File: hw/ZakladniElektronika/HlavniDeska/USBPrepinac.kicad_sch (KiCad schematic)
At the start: 1 part, among them U15 TS3USB3031

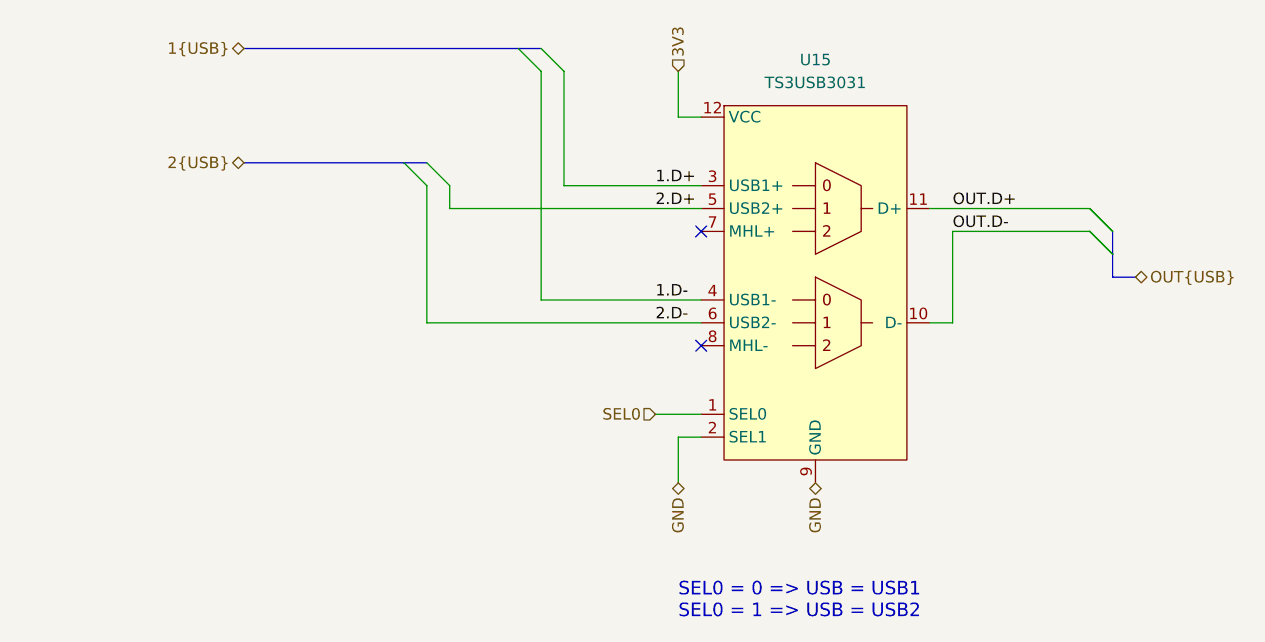
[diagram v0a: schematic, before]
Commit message: Hw PCB
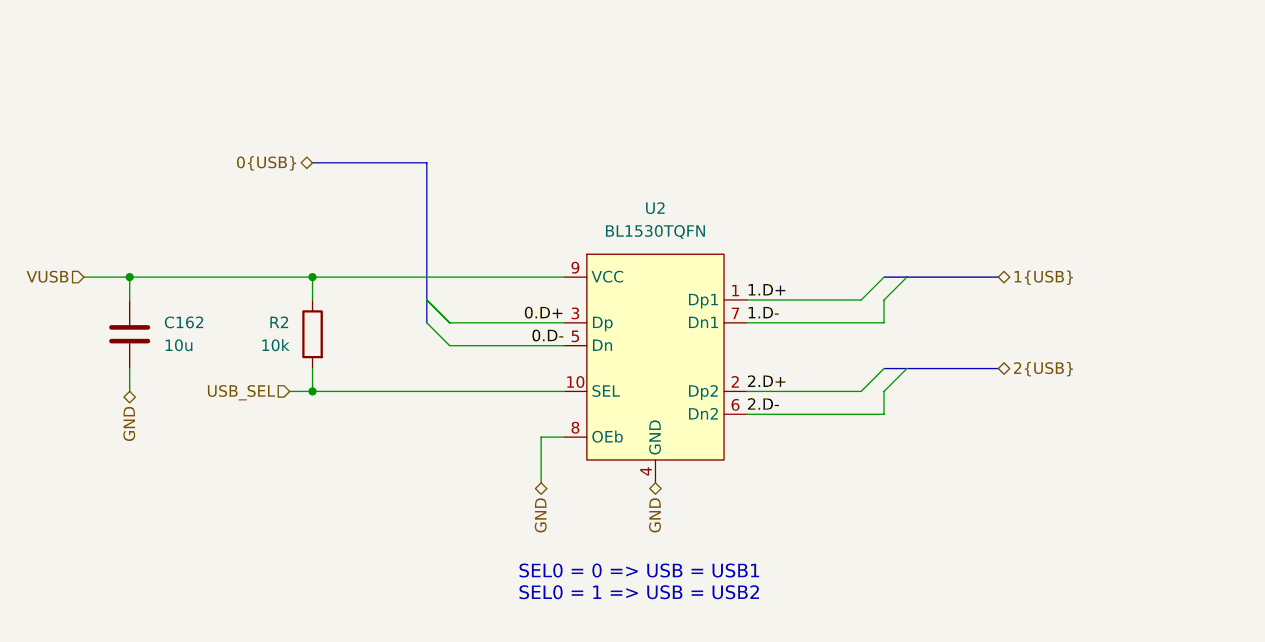
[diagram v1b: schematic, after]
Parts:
- removed U15: TS3USB3031, Package_DFN_QFN:Texas_X2QFN-12_1.6x1.6mm_P0.4mm, symbol RKL-DiscreteLogic:TS3USB3031
- added C162: 10u, Capacitor_SMD:C_0603_1608Metric, symbol Device:C
- added R2: 10k, Resistor_SMD:R_0402_1005Metric, symbol Device:R
- added U2: BL1530TQFN, Package_DFN_QFN:UQFN-10_1.4x1.8mm_P0.4mm, symbol RKL-Uncategorized:BL1530TQFN
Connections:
- net 1.D+: now also U2.1 (Dp1)
- net 1.D-: now also U2.7 (Dn1)
- net 2.D+: now also U2.2 (Dp2)
- net 2.D-: now also U2.6 (Dn2)
- net GND: now also C162.2, U2.4 (GND), U2.8 (OEb)
- new net 0.D+: U2.3 (Dp)
- new net 0.D-: U2.5 (Dn)
- new net USB_SEL: R2.2, U2.10 (SEL)
- new net VUSB: C162.1, R2.1, U2.9 (VCC)
- no-connect marks 2 -> 0
